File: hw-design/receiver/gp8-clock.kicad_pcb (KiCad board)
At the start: 2 copper layers, 102.3 x 50.9 mm, 65 parts, among them J1 CONN_01X01, J10 CONN_01X01, J11 CONN_01X01, J12 CONN_01X01, J2 CONN_01X01, J3 CONN_01X01, J4 CONN_01X01, J5 CONN_01X01, J6 CONN_01X01, J7 CONN_01X01, J8 CONN_01X01, J9 CONN_01X01, P1 CONN_01X03, P2 test-double, P3 CONN_01X04, P4 test-double, P5 test-double, P6 CONN_01X04, Q1 BC847, Q3 BC847, SW1 SW_PUSH, SW2 power, U1 TSOP39538, U2 weight-scale-lcd, U3 STM32F072CB / STM32F042C6, U4 usb-micro, U5 MCP73833, U6 MIC5504, U7 PCF85176T, Y1 8MHz

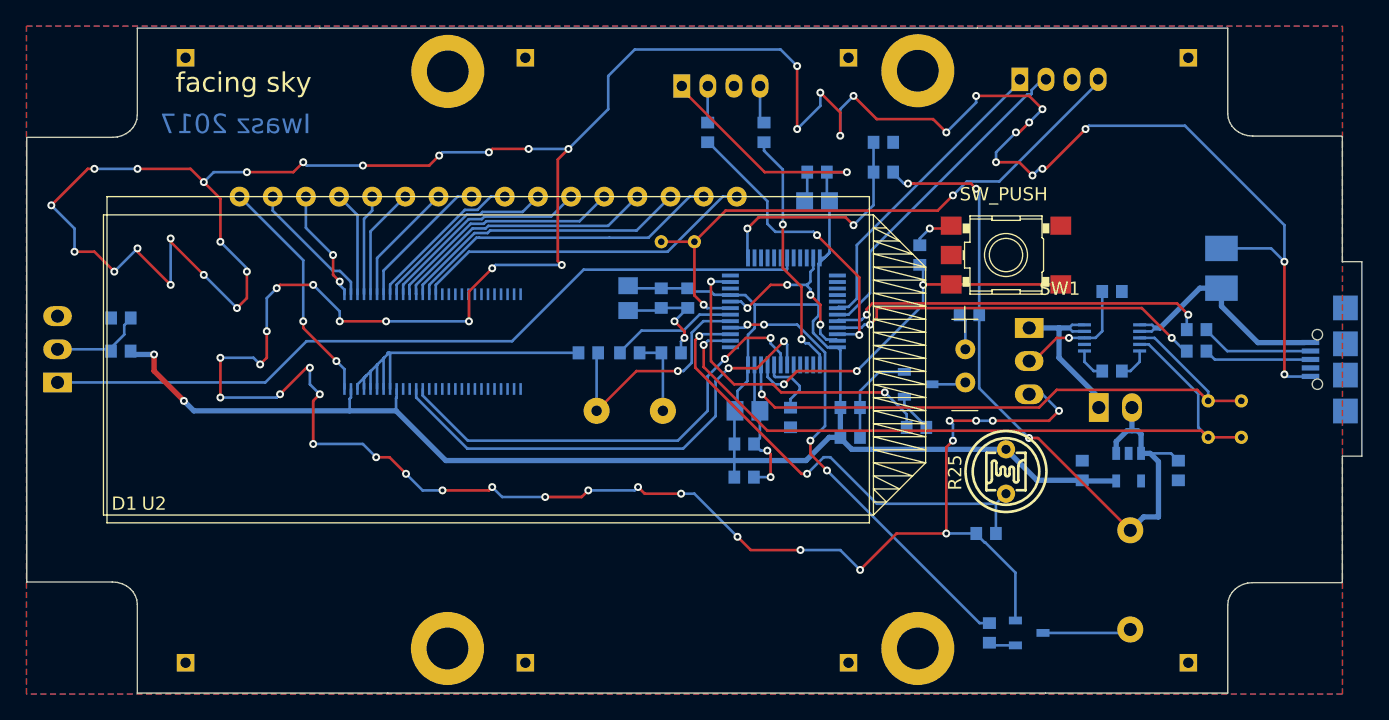
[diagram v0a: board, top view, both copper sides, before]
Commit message: Many changes
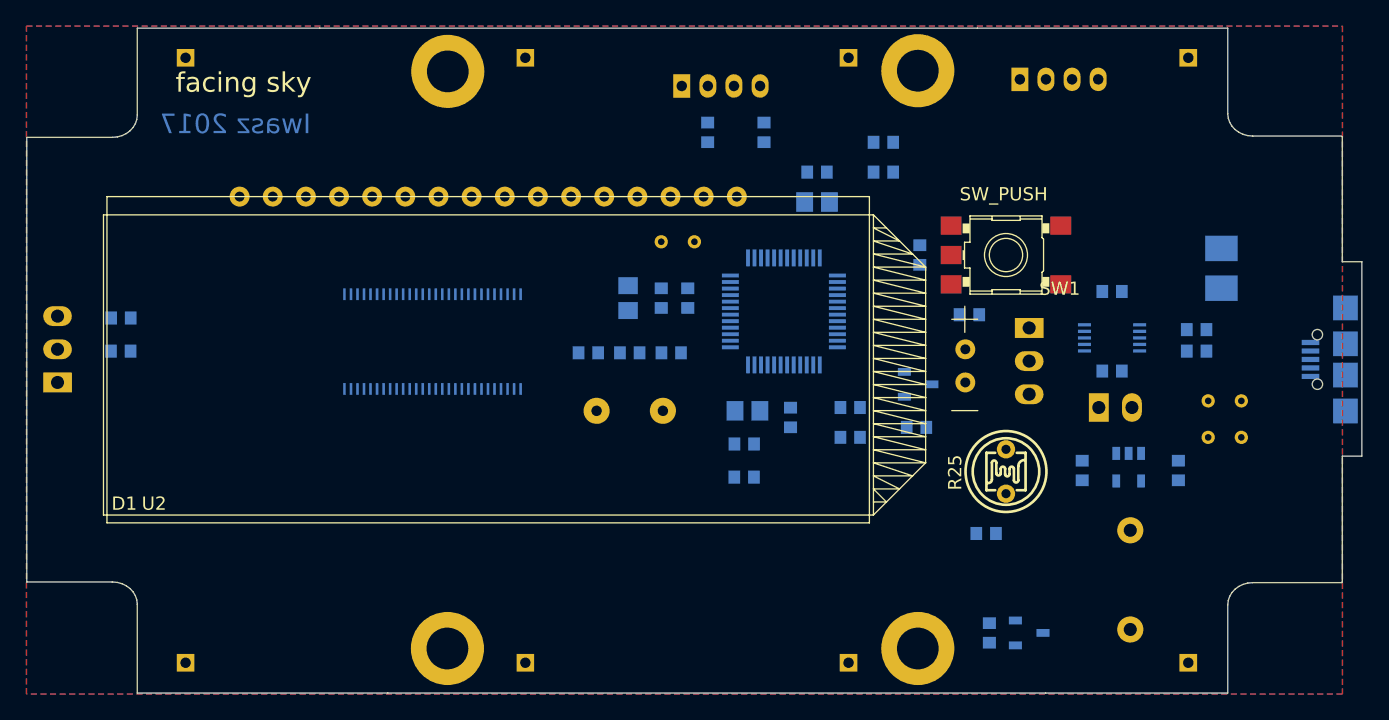
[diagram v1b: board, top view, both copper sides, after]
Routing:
- net GND: track 412.8 -> 0.00 mm, vias 77 -> 0
- net +3V3: track 154.6 -> 0.00 mm, vias 3 -> 0
- net /ir: track 60.4 -> 0.00 mm
- net /Sheet56372EC5/complete: track 57.0 -> 0.00 mm, vias 1 -> 0
- net +BATT: track 56.8 -> 0.00 mm, vias 3 -> 0
- net /Sheet56372EC5/progress: track 48.0 -> 0.00 mm, vias 1 -> 0
- net /nrst: track 46.1 -> 0.00 mm, vias 2 -> 0
- net /screen/scl: track 37.3 -> 0.00 mm, vias 2 -> 0
- net Net-(R25-Pad2): track 36.8 -> 0.00 mm, vias 2 -> 0
- net /screen/sda: track 35.8 -> 0.00 mm, vias 2 -> 0
- net /sound: track 35.6 -> 0.00 mm, vias 4 -> 0
- net Net-(C12-Pad1): track 29.3 -> 0.00 mm, vias 3 -> 0
- net Net-(R23-Pad2): track 29.3 -> 0.00 mm, vias 2 -> 0
- net Net-(R24-Pad2): track 29.2 -> 0.00 mm, vias 2 -> 0
- net Net-(U2-Pad16): track 26.6 -> 0.00 mm
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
